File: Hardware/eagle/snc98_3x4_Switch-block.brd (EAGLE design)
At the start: 57.5 x 84.2 mm, 67 parts

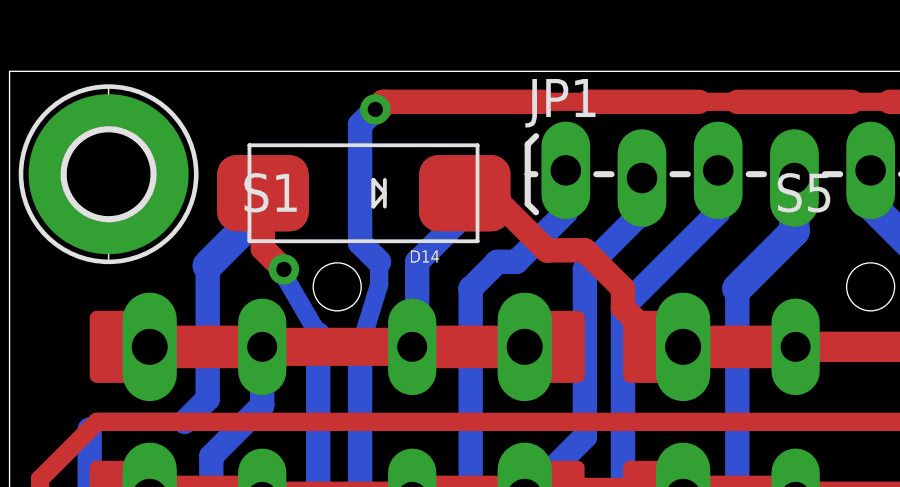
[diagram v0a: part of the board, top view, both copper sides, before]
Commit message: Debug_Level 13:  - Protokoll Statepoint
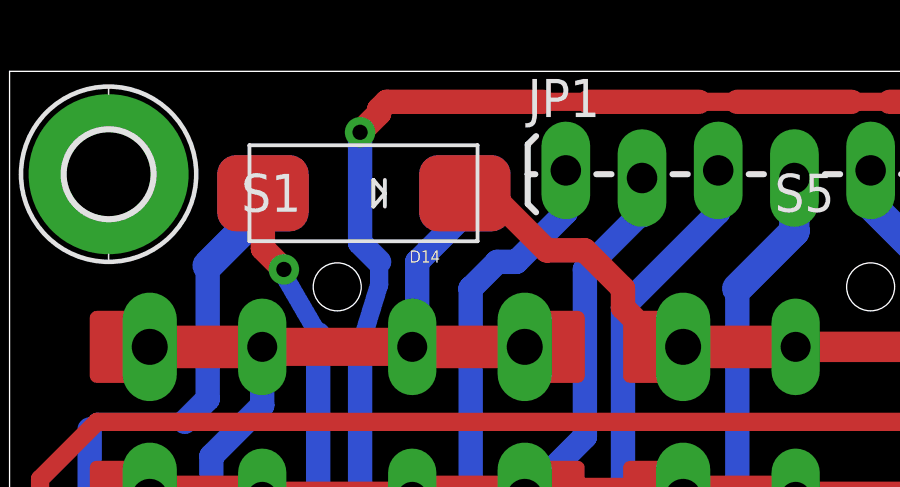
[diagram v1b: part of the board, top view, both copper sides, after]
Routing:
- net AREF: track 129.1 -> 128.6 mm
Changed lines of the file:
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@@
 <setting verticaltext="up"/>
 </settings>
-<grid distance="0.05" unitdist="inch" unit="inch" style="dots" multiple="1" display="yes" altdistance="0.005" altunitdist="inch" altunit="inch"/>
+<grid distance="10" unitdist="mil" unit="mil" style="dots" multiple="1" display="yes" altdistance="0.005" altunitdist="inch" altunit="inch"/>
 <layers>
 <layer number="1" name="Top" color="4" fill="1" visible="yes" active="yes"/>
@@
 <layer number="45" name="Holes" color="7" fill="1" visible="yes" active="yes"/>
 <layer number="46" name="Milling" color="3" fill="1" visible="no" active="yes"/>
-<layer number="47" name="Measures" color="7" fill="1" visible="yes" active="yes"/>
+<layer number="47" name="Measures" color="7" fill="1" visible="no" active="yes"/>
 <layer number="48" name="Document" color="7" fill="1" visible="no" active="yes"/>
 <layer number="49" name="Reference" color="7" fill="1" visible="no" active="yes"/>
@@
 </class>
 </classes>
-<designrules name="SparkFun_Iteadstudio_10mil *">
+<designrules name="OSHPark-8mil-2layer">
 <description language="en">&lt;b&gt;EAGLE Design Rules&lt;/b&gt;
 &lt;p&gt;
@@
 <param name="mtCopper" value="0.035mm 0.035mm 0.035mm 0.035mm 0.035mm 0.035mm 0.035mm 0.035mm 0.035mm 0.035mm 0.035mm 0.035mm 0.035mm 0.035mm 0.035mm 0.035mm"/>
 <param name="mtIsolate" value="1.5mm 0.15mm 0.2mm 0.15mm 0.2mm 0.15mm 0.2mm 0.15mm 0.2mm 0.15mm 0.2mm 0.15mm 0.2mm 0.15mm 0.2mm"/>
-<param name="mdWireWire" value="12mil"/>
-<param name="mdWirePad" value="12mil"/>
-<param name="mdWireVia" value="12mil"/>
-<param name="mdPadPad" value="12mil"/>
-<param name="mdPadVia" value="12mil"/>
-<param name="mdViaVia" value="12mil"/>
-<param name="mdSmdPad" value="12mil"/>
-<param name="mdSmdVia" value="12mil"/>
-<param name="mdSmdSmd" value="12mil"/>
+<param name="mdWireWire" value="8mil"/>
+<param name="mdWirePad" value="8mil"/>
+<param name="mdWireVia" value="8mil"/>
+<param name="mdPadPad" value="8mil"/>
+<param name="mdPadVia" value="8mil"/>
+<param name="mdViaVia" value="8mil"/>
+<param name="mdSmdPad" value="8mil"/>
+<param name="mdSmdVia" value="8mil"/>
+<param name="mdSmdSmd" value="8mil"/>
 <param name="mdViaViaSameLayer" value="8mil"/>
 <param name="mnLayersViaInSmd" value="2"/>
-<param name="mdCopperDimension" value="0.5mm"/>
+<param name="mdCopperDimension" value="8mil"/>
 <param name="mdDrill" value="8mil"/>
 <param name="mdSmdStop" value="0mil"/>
 <param name="msWidth" value="10mil"/>
-<param name="msDrill" value="20mil"/>
+<param name="msDrill" value="15mil"/>
 <param name="msMicroVia" value="9.99mm"/>
 <param name="msBlindViaRatio" value="0.5"/>
@@
 <param name="mlMinCreamFrame" value="0mil"/>
 <param name="mlMaxCreamFrame" value="0mil"/>
-<param name="mlViaStopLimit" value="25mil"/>
+<param name="mlViaStopLimit" value="20mil"/>
 <param name="srRoundness" value="0"/>
 <param name="srMinRoundness" value="0mil"/>
@@
 <wire x1="14.097" y1="67.691" x2="12.573" y2="67.691" width="0.6096" layer="16"/>
 <wire x1="12.573" y1="67.691" x2="12.319" y2="67.945" width="0.6096" layer="16"/>
-<wire x1="11.684" y1="82.423" x2="12.192" y2="82.931" width="0.8128" layer="16"/>
-<via x="12.192" y="82.931" extent="1-16" drill="0.508"/>
-<wire x1="12.192" y1="82.931" x2="12.319" y2="82.931" width="0.8128" layer="1"/>
+<via x="11.684" y="82.169" extent="1-16" drill="0.508"/>
 <wire x1="12.319" y1="82.931" x2="12.573" y2="83.185" width="0.8128" layer="1"/>
 <wire x1="38.989" y1="81.915" x2="38.989" y2="81.026" width="0.8128" layer="1"/>
@@
 <wire x1="22.987" y1="83.185" x2="19.304" y2="83.185" width="0.8128" layer="1"/>
 <wire x1="19.304" y1="83.185" x2="17.78" y2="83.185" width="0.6096" layer="1"/>
-<wire x1="17.78" y1="83.185" x2="12.446" y2="83.185" width="0.8128" layer="1"/>
-<wire x1="12.446" y1="83.185" x2="12.192" y2="82.931" width="0.8128" layer="1"/>
-<wire x1="11.684" y1="82.423" x2="11.684" y2="78.486" width="0.8128" layer="16"/>
+<wire x1="17.78" y1="83.185" x2="12.573" y2="83.185" width="0.8128" layer="1"/>
+<wire x1="11.684" y1="82.169" x2="11.684" y2="78.486" width="0.8128" layer="16"/>
 <wire x1="11.684" y1="78.486" x2="12.319" y2="77.851" width="0.8128" layer="16"/>
 <wire x1="12.319" y1="77.851" x2="12.319" y2="77.089" width="0.6096" layer="16"/>
@@
 <wire x1="16.002" y1="43.434" x2="31.75" y2="43.434" width="0.8128" layer="1"/>
 <wire x1="12.319" y1="67.945" x2="11.684" y2="69.80620625" width="0.6096" layer="16"/>
+<wire x1="12.319" y1="82.931" x2="12.319" y2="82.804" width="0.8128" layer="1"/>
+<wire x1="12.319" y1="82.804" x2="11.684" y2="82.169" width="0.8128" layer="1"/>
 </signal>
 <signal name="A_1">

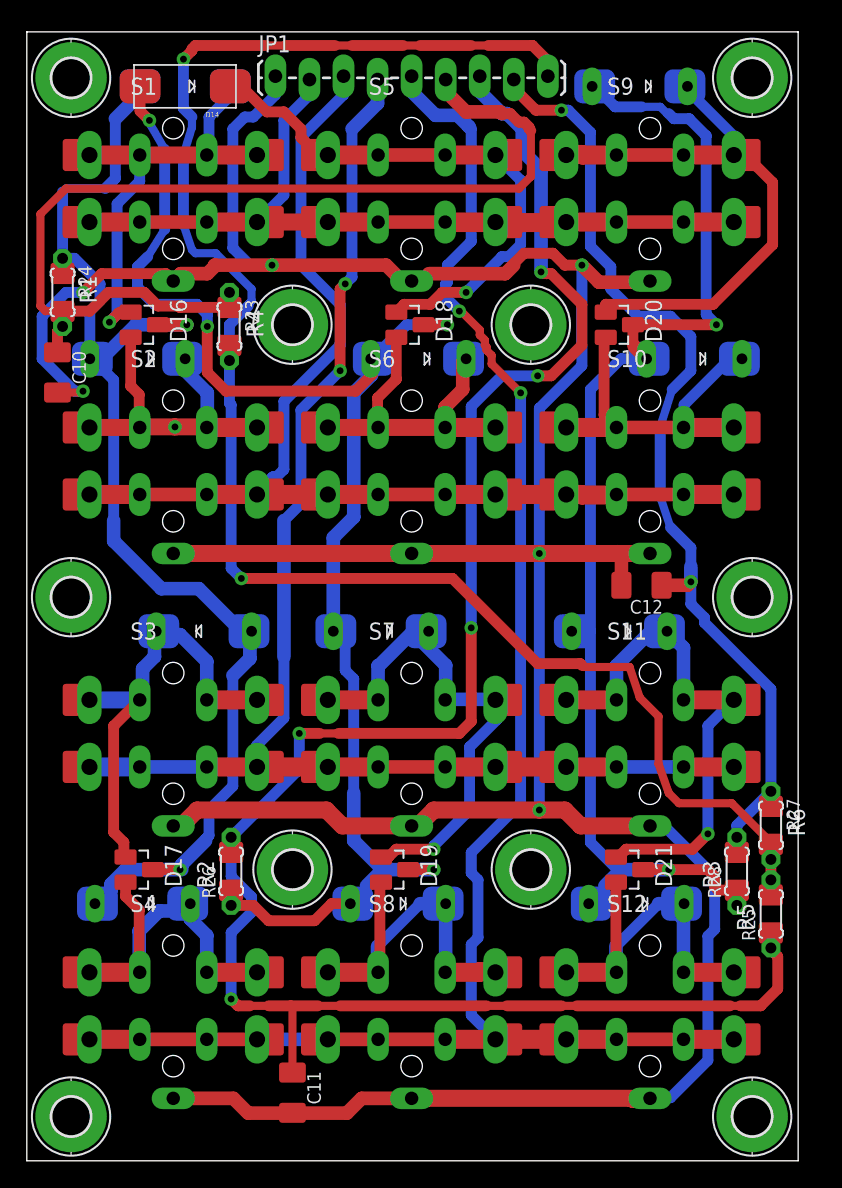
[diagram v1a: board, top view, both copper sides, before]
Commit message: Debuglevel 13 - Protokoll Statepoint
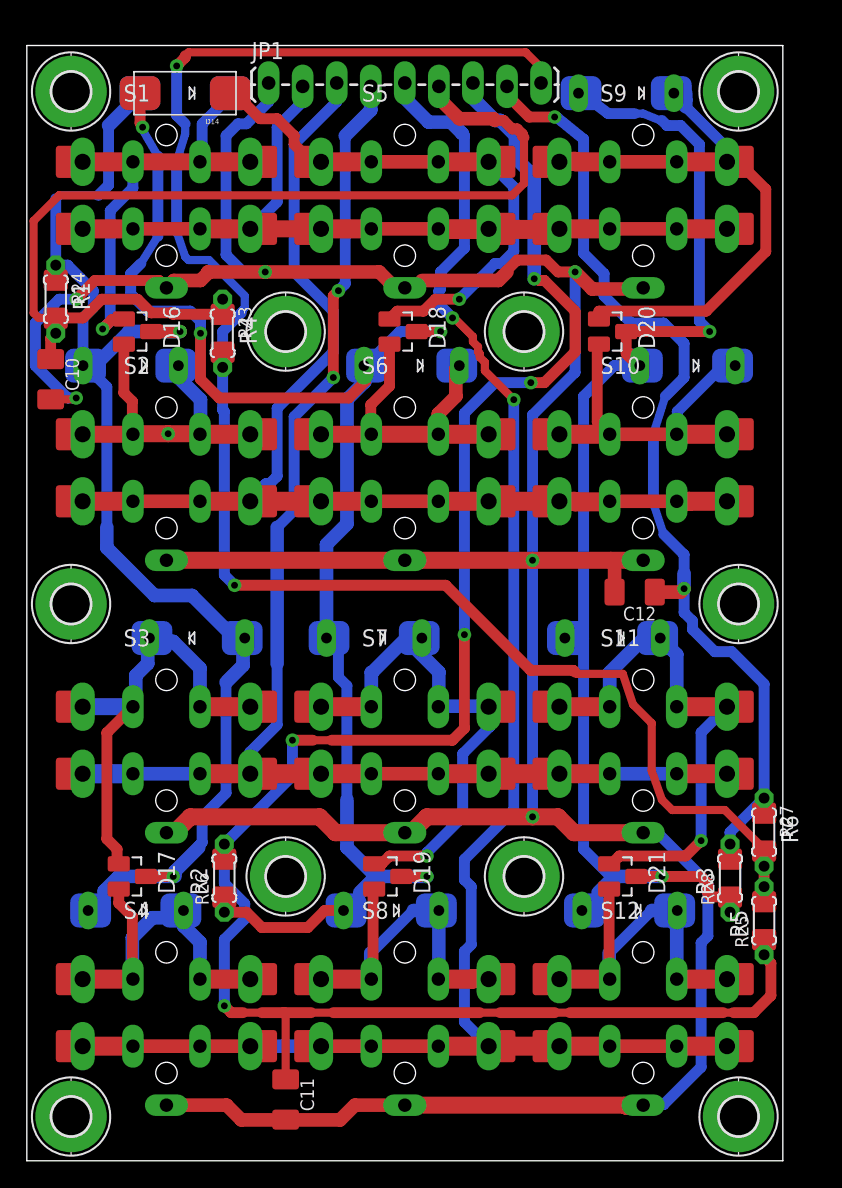
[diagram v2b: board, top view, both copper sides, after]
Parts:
- moved H8 1.44 mm to (53.1, 79.8)
- moved D15 1.14 mm to (44.7, 79.6)
- moved D6 1.14 mm to (44.7, 79.6)
- moved H9 1.14 mm to (53.1, 41.5)
- moved H1 1.02 mm to (3.30, 79.8)
- moved H10 1.02 mm to (53.1, 3.30)
- moved JP1 0.72 mm to (18.0, 80.3)
- moved C12 0.72 mm to (45.3, 42.4)
- moved H4 0.72 mm to (19.3, 61.8)
- moved S10 0.72 mm to (46.0, 51.7)
- moved S6 0.72 mm to (28.2, 51.7)
- moved D12 0.72 mm to (7.75, 59.3)
- moved D24 0.72 mm to (12.7, 39.0)
- moved D27 0.72 mm to (7.75, 59.3)
- moved D29 0.72 mm to (12.7, 39.0)
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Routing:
- net N$16: track 45.0 -> 45.9 mm
- net A3: track 74.3 -> 75.0 mm
- net N$24: track 42.1 -> 41.6 mm
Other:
- board size 57.5 x 84.2 mm -> 56.4 x 83.2 mm
